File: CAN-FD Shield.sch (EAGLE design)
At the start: 37 parts, among them J2 JUMPER-3P-SHORT, J3 JUMPER-3P-SHORT, J4 JUMPER-3P-SHORT, J5 JUMPER-3P-SHORT, U5 MCP2517FD, U6 MCP2542, X2 20MHz

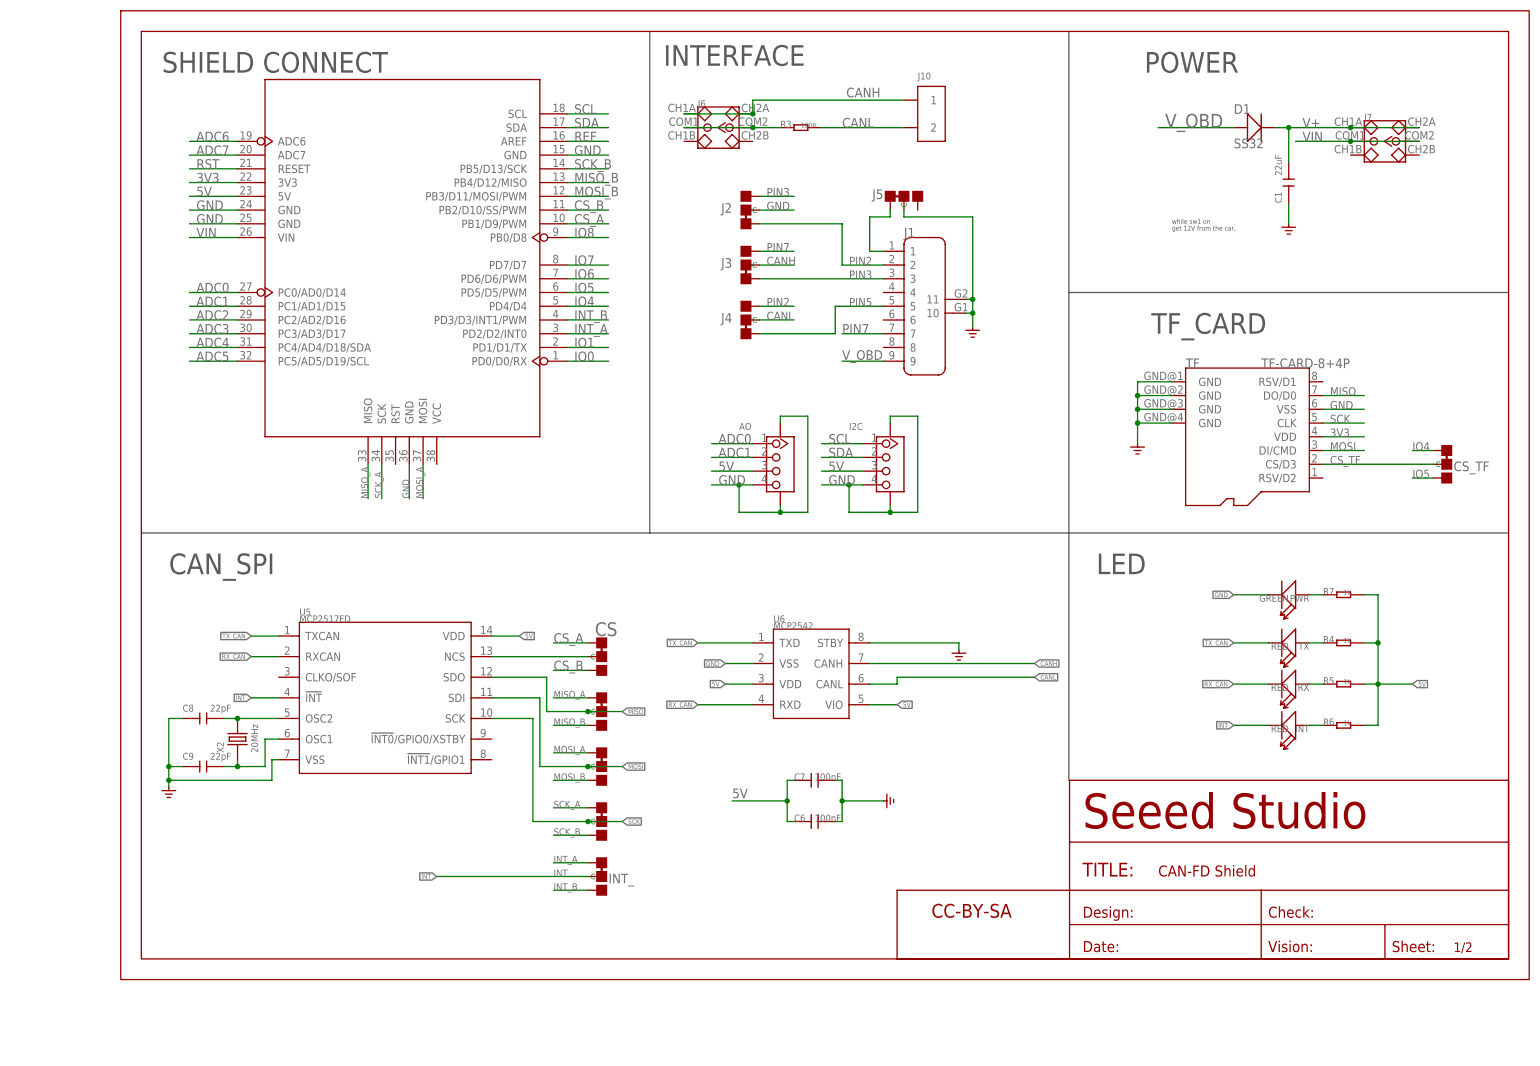
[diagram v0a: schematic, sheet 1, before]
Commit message: update
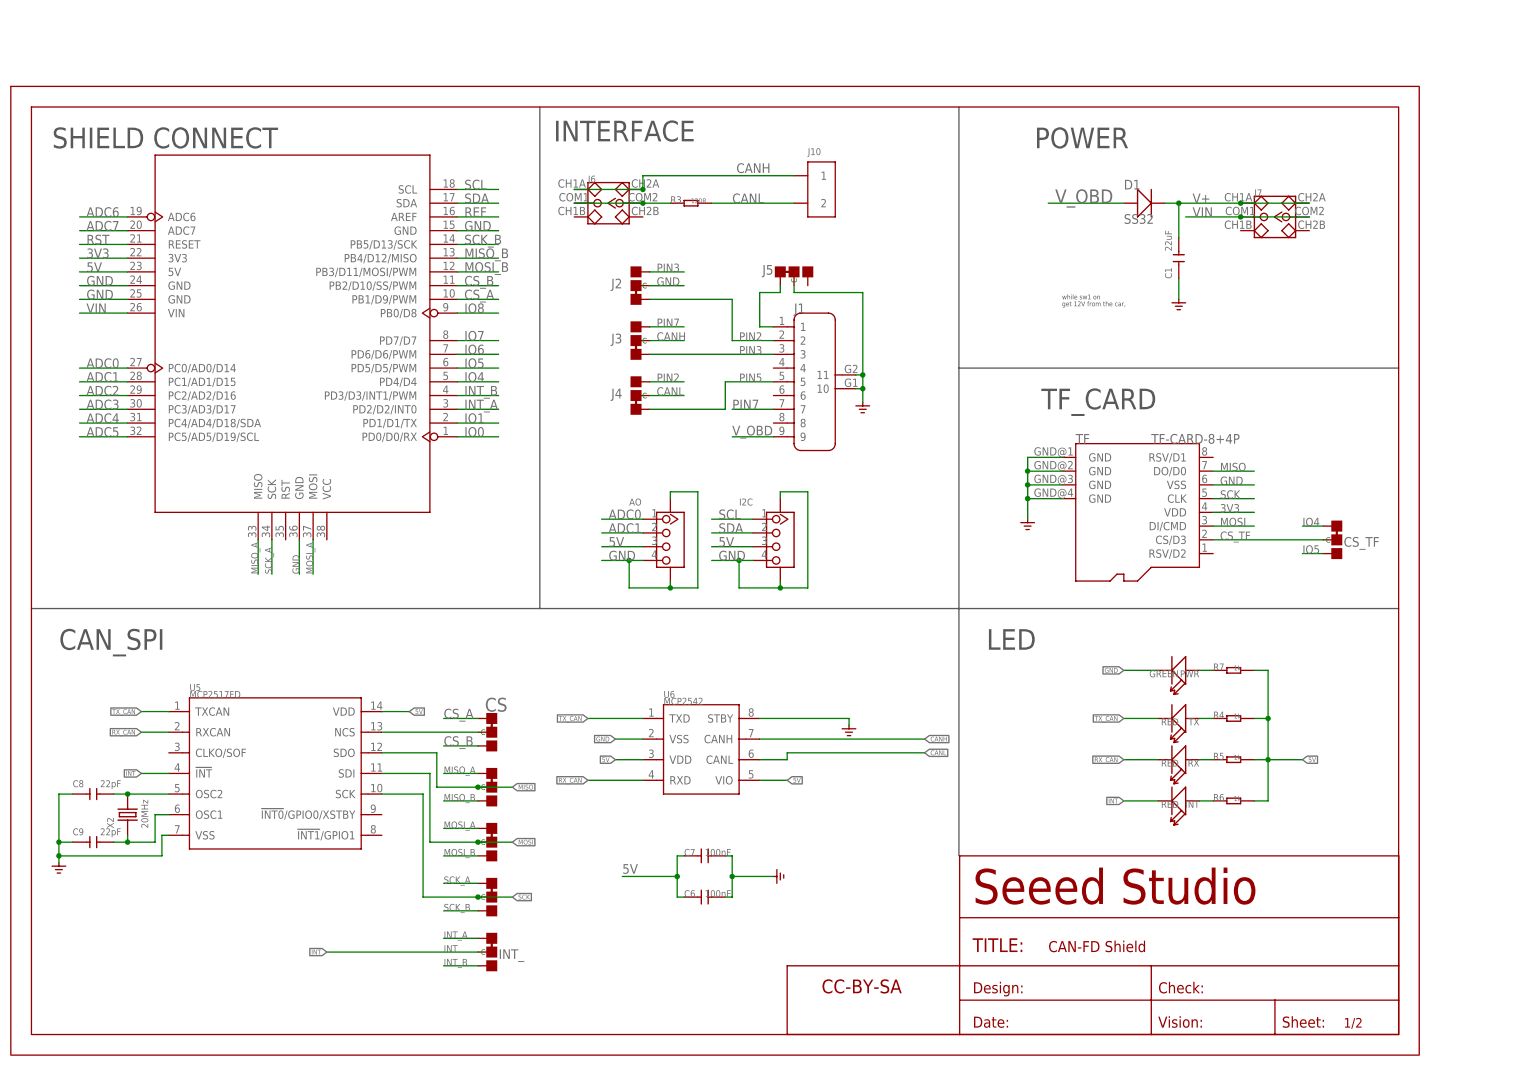
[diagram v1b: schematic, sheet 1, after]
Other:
- moved on the sheet: AO, C1, C6, C7, C8, C9, CS, CS_TF, D1, I2C, INT, INT_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
